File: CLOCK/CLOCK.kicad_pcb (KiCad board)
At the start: 2 copper layers, 140 x 90 mm, 60 parts, among them J1 Conn_01x06, J3 Conn_02x03_Odd_Even, J4 Conn_01x05, J5 Conn_01x03, SW1 Omron_B3F_SPST, SW2 Omron_B3F_SPST, SW3 Omron_B3F_SPST, SW4 Omron_B3F_SPST, SW5 Omron_B3F_SPST, U1 ATmega328-PU, U2 L7805, U3 DS1307_DIP-8, U4 MAX7219, U5 MAX7219, U6 MAX7219, U7 MAX7219, U8 ADT7410, Y1 Crystal_16MHz, Y2 Crystal_32768Hz

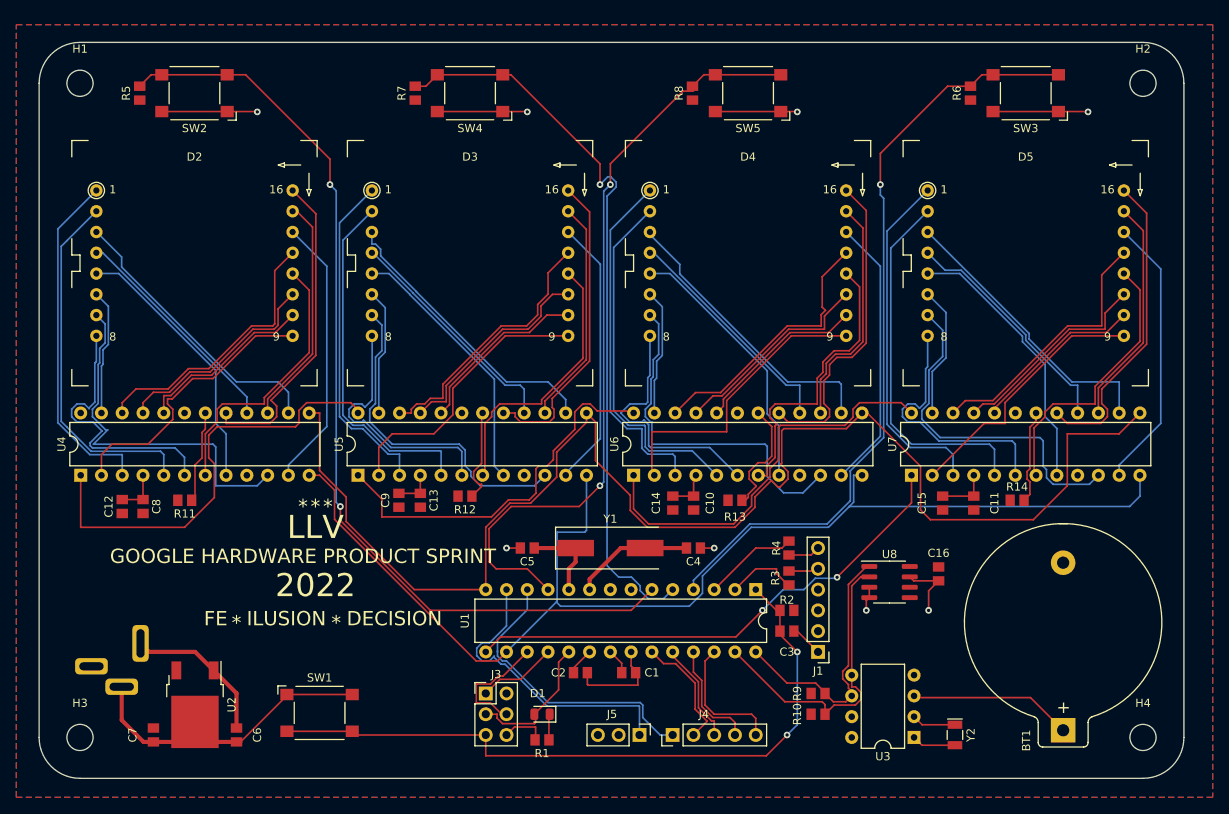
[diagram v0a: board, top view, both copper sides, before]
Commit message: GERBER OUT
LLV-BOARD
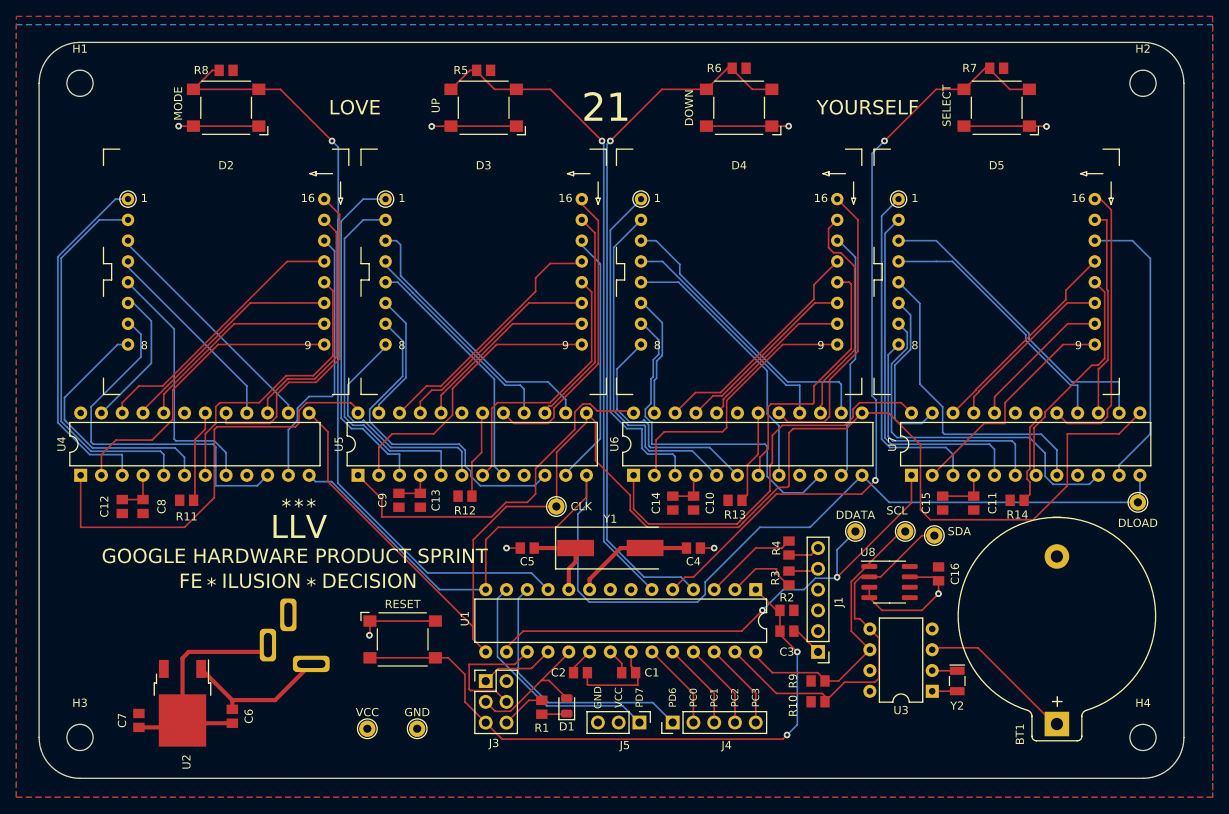
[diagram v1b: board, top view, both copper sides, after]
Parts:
- added CLK: TestPoint, footprints:TestPoint_THTPad_D2.0mm_Drill1.0mm, F.Cu at (143.3, 111.8)
- added DDATA: TestPoint, footprints:TestPoint_THTPad_D2.0mm_Drill1.0mm, F.Cu at (179.8, 114.8)
- added DLOAD: TestPoint, footprints:TestPoint_THTPad_D2.0mm_Drill1.0mm, F.Cu at (214.4, 111.3)
- added G***: LOGO, footprints:HPS_logo, B.Cu at (117.3, 116.3)
- added GND: TestPoint, footprints:TestPoint_THTPad_D2.0mm_Drill1.0mm, F.Cu at (126.2, 138.9)
- added SCL: TestPoint, footprints:TestPoint_THTPad_D2.0mm_Drill1.0mm, F.Cu at (185.9, 114.8)
- added SDA: TestPoint, footprints:TestPoint_THTPad_D2.0mm_Drill1.0mm, F.Cu at (189.5, 115.3)
- added VCC: TestPoint, footprints:TestPoint_THTPad_D2.0mm_Drill1.0mm, F.Cu at (120.1, 138.9)
- moved R7 71.2 mm to (197.1, 58.2), turned to 180 degrees
- moved SELECT 64.4 mm to (197.1, 63.0)
- moved MODE 63.9 mm to (102.9, 63.0)
- moved R8 57.1 mm to (102.9, 58.4), turned to 180 degrees
- moved R5 42.2 mm to (134.4, 58.4), turned to 180 degrees
- moved UP 35.4 mm to (134.4, 63.0)
- moved DOWN 35.1 mm to (165.6, 63.0)
- moved R6 28.5 mm to (165.6, 58.2), turned to 180 degrees
- moved REF**1 24.4 mm to (113.3, 127.5), turned to 90 degrees
- moved RESET 13.6 mm to (124.5, 128.0)
- moved Y2 6.61 mm to (192.3, 133.1)
- moved U3 6.06 mm to (189.2, 134.4)
- moved D2 4.01 mm to (102.9, 83.1)
- moved R1 3.99 mm to (141.5, 136.3), turned to 90 degrees
- moved D5 3.71 mm to (197.1, 83.1)
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- renumbered SW3 to DOWN, SW5 to MODE, SW1 to RESET, SW4 to SELECT, SW2 to UP
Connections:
- R12 pad 1: VCC -> Net-(U5-Pad18)
- R12 pad 2: Net-(R12-Pad2) -> VCC
- R13 pad 1: VCC -> Net-(U6-Pad18)
- R13 pad 2: Net-(R13-Pad2) -> VCC
- R14 pad 1: VCC -> Net-(U7-Pad18)
- R14 pad 2: Net-(R14-Pad2) -> VCC
- U1 pad 14: CLK -> DLOAD
- U1 pad 15: DIN -> CLK
- U1 pad 16: CS -> DDATA
- U4 pad 12: CS -> DLOAD
- U4 pad 24: D_OUT -> unconnected-(U4-Pad24)
- U5 pad 12: CS -> DLOAD
- U5 pad 18: Net-(R12-Pad2) -> Net-(U5-Pad18)
- U6 pad 12: CS -> DLOAD
- U6 pad 18: Net-(R13-Pad2) -> Net-(U6-Pad18)
- U7 pad 1: DIN -> DDATA
- U7 pad 12: CS -> DLOAD
- U7 pad 18: Net-(R14-Pad2) -> Net-(U7-Pad18)
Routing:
- net CS: track 149.7 -> 0.00 mm
- net DLOAD: track 0.00 -> 146.4 mm
- net DDATA: track 0.00 -> 67.3 mm, vias 0 -> 2
- net DIN: track 63.0 -> 0.00 mm, vias 2 -> 0
- net BTN_UP: track 116.5 -> 80.5 mm, vias 2 -> 1
- net Net-(R13-Pad2): track 14.3 -> 0.00 mm
- net Net-(R12-Pad2): track 11.7 -> 0.00 mm
- net Net-(U7-Pad18): track 0.00 -> 11.6 mm
- net Net-(R14-Pad2): track 11.6 -> 0.00 mm
- net Net-(U6-Pad18): track 0.00 -> 11.5 mm
- net Net-(U5-Pad18): track 0.00 -> 10.7 mm
- net SDA: track 37.2 -> 47.1 mm
- net CLK: track 171.5 -> 180.3 mm
- net BTN_DWN: track 94.5 -> 86.6 mm
- net RESET: track 85.6 -> 78.0 mm
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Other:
- board text added: "21"
- board text added: "AMOR"
- board text added: "FAMILIA"
- board text added: "GILBERTO*LAURA*BERNICE"
- board text added: "GND"
- board text added: "HONOR"
- board text added: "JUNE-AUGUST 2022"
- board text added: "LOVE"
- board text added: "LUJAN VILLASANA"
- board text added: "PANUCO,ZACATECAS"
- board text added: "PC0"
- board text added: "PC1"
- board text added: "PC2"
- board text added: "PC3"
- board text added: "PD6"
- board text added: "PD7"
- board text added: "RESPETO"
- board text added: "RIVERSIDE,CALIFORNIA"
- board text added: "TRUTH,LOYALTY,WISDOM"
- board text added: "VCC"
- board text added: "YOURSELF"
- board text removed: "2022"
